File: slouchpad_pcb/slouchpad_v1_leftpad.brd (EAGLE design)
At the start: 41 x 69 mm, 13 parts

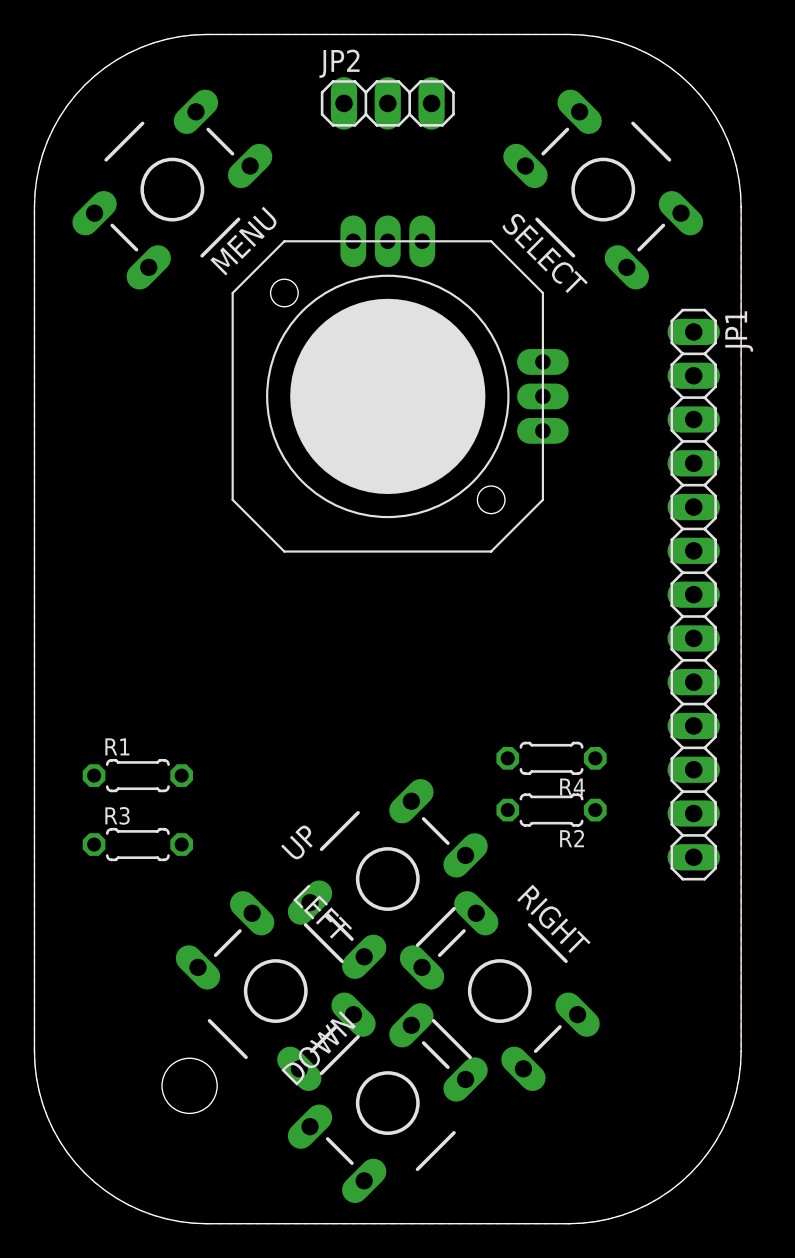
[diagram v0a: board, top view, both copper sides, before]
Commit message: Finished board layouts
Cleaned up schematics
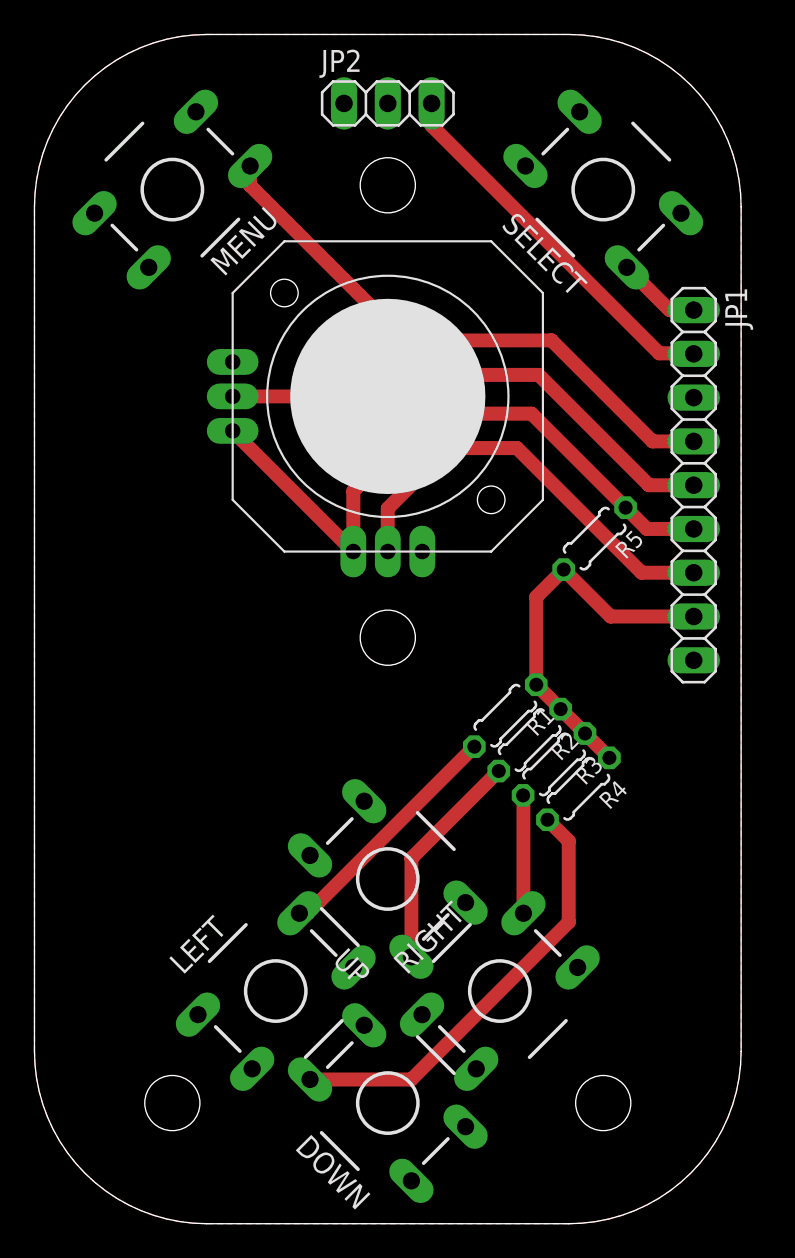
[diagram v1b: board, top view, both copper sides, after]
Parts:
- added R5: 10K, resistor:0204/5
- JP1: device pinhead:1X13 -> pinhead:1X09
- R1: value (none) -> 10K
- R2: value (none) -> 22K
- R3: value (none) -> 33K
- R4: value (none) -> 47K
- moved R3 24.6 mm to (30.1, 26.6), turned to 225 degrees
- moved R1 21.6 mm to (27.3, 29.5), turned to 225 degrees
- moved JP1 6.35 mm to (38.2, 42.9)
- moved R2 4.25 mm to (28.7, 28.1), turned to 225 degrees
- moved R4 2.36 mm to (31.6, 25.2), turned to 225 degrees
- turned DOWN to 135 degrees
- turned JOY1 to 180 degrees
- turned LEFT to 45 degrees
- turned RIGHT to 45 degrees
- turned UP to 135 degrees
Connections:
- removed net A: JP1.7
- removed net B: JP1.8
- removed net C: JP1.9
- removed net DOWN: DOWN.1, DOWN.2, R2.2
- removed net LEFT: LEFT.1, LEFT.2, R3.2
- removed net RIGHT: R4.2, RIGHT.1, RIGHT.2
- removed net START: JP1.1
- removed net UP: R1.2, UP.1, UP.2
- removed net X: JP1.6
- removed net Y: JP1.5
- removed net Z: JP1.4
- new net DPAD: JP1.8, R1.1, R2.1, R3.1, R4.1, R5.2
- new net N$1: JP1.2, JP2.3
- new net N$4: R3.2, RIGHT.1, RIGHT.2
- new net N$5: DOWN.1, DOWN.2, R4.2
- new net N$6: R2.2, UP.1, UP.2
- net GND: now also JP1.9; no longer JP1.13
- net JOYX: now also JP1.7; no longer JP1.12
- net JOYY: now also JP1.5; no longer JP1.10
- net MENU: now also JP1.4
- net N$2: now also JP1.3; no longer JP1.2
- net N$3: now also LEFT.1, LEFT.2, R1.2; no longer JP1.3, JP2.3
- net SELECT: now also JP1.1
- net VCC: now also JP1.6, R5.1; no longer JP1.11
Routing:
- net VCC: track 0.00 -> 37.8 mm
- net MENU: track 0.00 -> 33.0 mm
- net JOYY: track 0.00 -> 29.9 mm
- net N$5: track 0.00 -> 25.2 mm
- net JOYX: track 0.00 -> 24.7 mm
- net DPAD: track 0.00 -> 22.0 mm
- net N$1: track 0.00 -> 22.0 mm
- net N$3: track 0.00 -> 14.2 mm
- net N$6: track 0.00 -> 12.9 mm
- net N$4: track 0.00 -> 6.85 mm
- net SELECT: track 0.00 -> 4.91 mm
